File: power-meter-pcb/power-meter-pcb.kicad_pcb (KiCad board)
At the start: 2 copper layers, 28.7 x 55.6 mm, 65 parts, among them J1 Crank interconnect, J2 Debug, J3 USB4120-03-C_REVA, J4 Battery_Cell, J5 Side A, J6 Side B, Q1 AS2302, Q2 AS2302, Q3 AS2302, SW1 EN, SW2 BOOT, U1 ESP32-S3-WROOM-1, U2 P3T1755, U3 MCP73831-2-OT, U4 TPD3E001DRLR, U5 S-8261AAJMD-G2JT2U, U6 TPS63031DSK, U7 ADS1232IPW

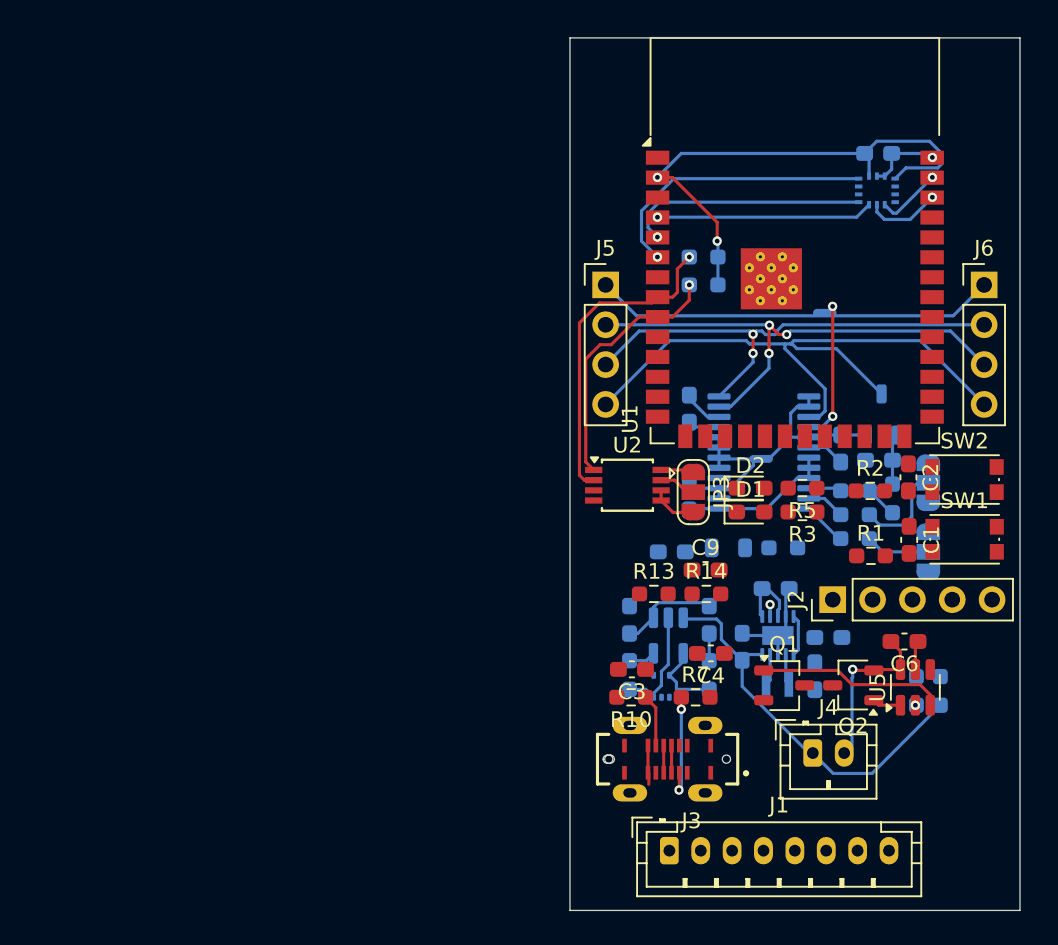
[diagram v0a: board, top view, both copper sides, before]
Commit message: Improved board outline, in the middle of layout changes
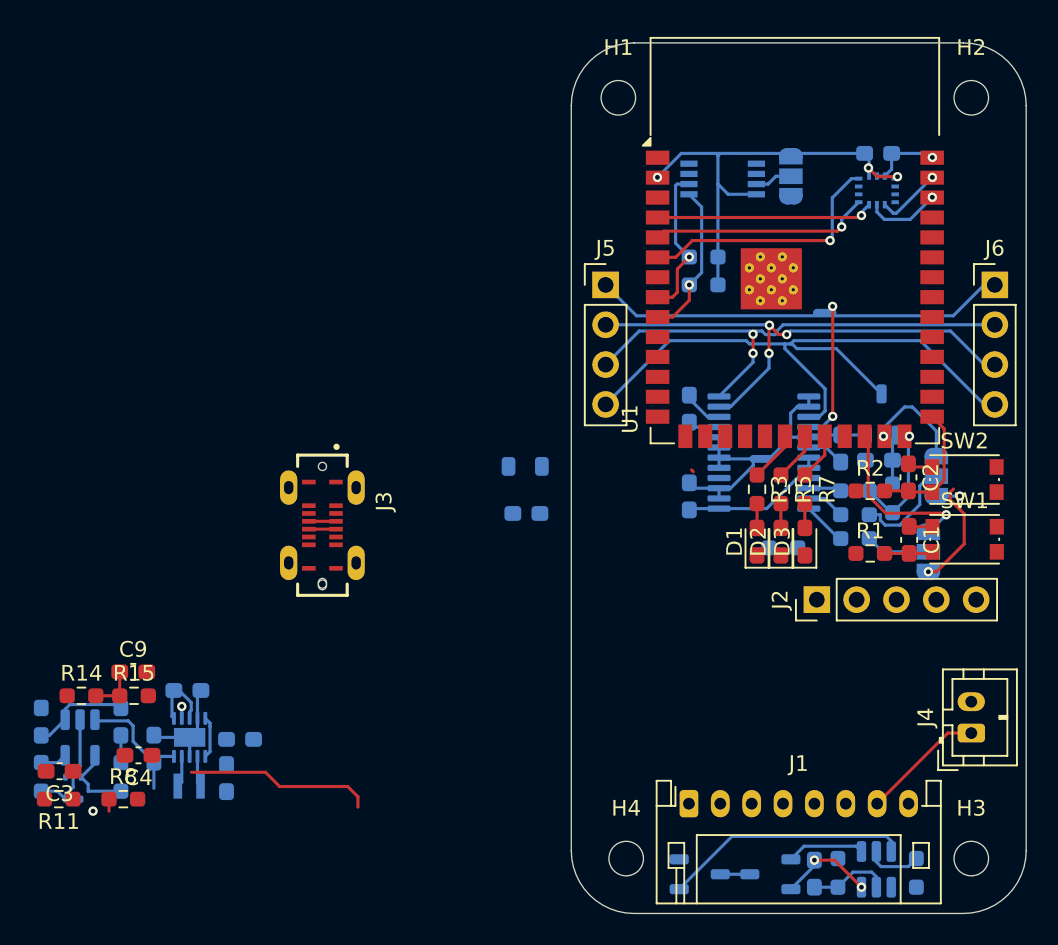
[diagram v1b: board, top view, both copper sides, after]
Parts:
- added D3: LED, LED_SMD:LED_0603_1608Metric_Pad1.05x0.95mm_HandSolder, F.Cu at (135.9, 75.3)
- added H1: MountingHole, MountingHole:MountingHole_2.2mm_M2, F.Cu at (124.0, 47.0)
- added H2: MountingHole, MountingHole:MountingHole_2.2mm_M2, F.Cu at (146.5, 47.0)
- added H3: MountingHole, MountingHole:MountingHole_2.2mm_M2, F.Cu at (146.5, 95.5)
- added H4: MountingHole, MountingHole:MountingHole_2.2mm_M2, F.Cu at (124.5, 95.5)
- added R7: 150, Resistor_SMD:R_0603_1608Metric_Pad0.98x0.95mm_HandSolder, F.Cu at (135.9, 72.0)
- C6, JP3, Q1, Q2, U2, U5: moved to B.Cu
- J1: footprint Connector_JST:JST_PH_B8B-PH-K_1x08_P2.00mm_Vertical -> Connector_JST:JST_PH_S8B-PH-K_1x08_P2.00mm_Horizontal
- moved C10 38.1 mm to (99.0, 90.4)
- moved C5 38.1 mm to (94.4, 88.5)
- moved D4 38.1 mm to (92.3, 86.8)
- moved D5 38.1 mm to (87.2, 86.8)
- moved R10 38.1 mm to (92.3, 90.3)
- moved R9 38.1 mm to (87.2, 90.3)
- moved U3 38.1 mm to (89.7, 87.8)
- moved U4 38.1 mm to (89.2, 91.0)
- moved C7 38.1 mm to (96.5, 84.8)
- moved C8 38.1 mm to (99.9, 87.9)
- moved L1 38.1 mm to (96.6, 90.9)
- moved U6 38.1 mm to (96.7, 87.8)
- moved C3 37.1 mm to (88.4, 89.9)
- moved R8 37.1 mm to (92.4, 91.7)
- moved C4 37.1 mm to (93.4, 88.9)
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- renumbered D3 to D4, D4 to D5, R9 to R10, R10 to R11, R11 to R12, R12 to R13, R13 to R14, R14 to R15, R15 to R16, R16 to R17, R17 to R18, R18 to R19, R19 to R20, R7 to R8, R8 to R9
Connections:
- net /USB and charging/Battery voltage renamed /USB and power supply/Battery voltage
- net /USB and charging/Charging renamed /USB and power supply/Charging
- J3 pad A6: /USB and charging/USB.DP -> /USB and power supply/USB.D_P
- J3 pad A7: /USB and charging/USB.DN -> /USB and power supply/USB.D_N
- J3 pad B6: /USB and charging/USB.DN -> /USB and power supply/USB.D_N
- J3 pad B7: /USB and charging/USB.DP -> /USB and power supply/USB.D_P
- U1 pad 13: /USB and charging/USB.DN -> /USB and power supply/USB.D_N
- U1 pad 14: /USB and charging/USB.DP -> /USB and power supply/USB.D_P
- U1 pad 20: unconnected-(U1-IO12-Pad20) -> /LED1
- U1 pad 21: unconnected-(U1-IO13-Pad21) -> /LED2
- U1 pad 22: unconnected-(U1-IO14-Pad22) -> /LED3
- U1 pad 26: unconnected-(U1-IO45-Pad26) -> /AMP_PWDN
- U1 pad 31: /LED1 -> /AMP1.DOUT
- U1 pad 32: /LED2 -> /AMP1.SCLK
- U1 pad 33: /AMP1.DOUT -> unconnected-(U1-IO40-Pad33)
- U1 pad 34: /AMP1.SCLK -> unconnected-(U1-IO41-Pad34)
- U1 pad 35: /AMP_PWDN -> unconnected-(U1-IO42-Pad35)
- U4 pad 1: /USB and charging/USB.DP -> /USB and power supply/USB.DP
- U4 pad 2: /USB and charging/USB.DN -> /USB and power supply/USB.DN
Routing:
- net Net-(Q1-G): track 11.9 -> 27.6 mm
- net /AMP2.DOUT: track 0.00 -> 10.9 mm, vias 0 -> 1
- net /I2C.SDA: track 20.4 -> 10.3 mm, vias 1 -> 2
- net +BATT: track 25.3 -> 16.4 mm
- net /BOOT: track 0.00 -> 8.51 mm
- net +3.3V: track 48.5 -> 41.5 mm, vias 2 -> 3
- net /AMP1.DOUT: track 0.00 -> 6.97 mm, vias 0 -> 1
- net /AMP2.SCLK: track 0.00 -> 6.73 mm, vias 0 -> 1
- net /I2C.SCL: track 16.4 -> 9.89 mm
- net Net-(J3-CC1): track 7.09 -> 0.76 mm, vias 2 -> 0
- net /AMP_PWDN: track 2.06 -> 7.38 mm, vias 0 -> 1
- net Net-(J4--): track 10.5 -> 6.19 mm, vias 1 -> 2
- net Net-(U5-VM): track 0.07 -> 3.55 mm, vias 1 -> 0
- net Net-(J3-CC2): track 3.35 -> 0.00 mm
- net Net-(U5-VDD): track 1.86 -> 5.14 mm
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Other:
- board size 28.7 x 55.6 mm -> 29 x 55.5 mm
- board text added: "${REFERENCE}"
